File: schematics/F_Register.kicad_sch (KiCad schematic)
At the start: 5 parts, among them U1 74LS377

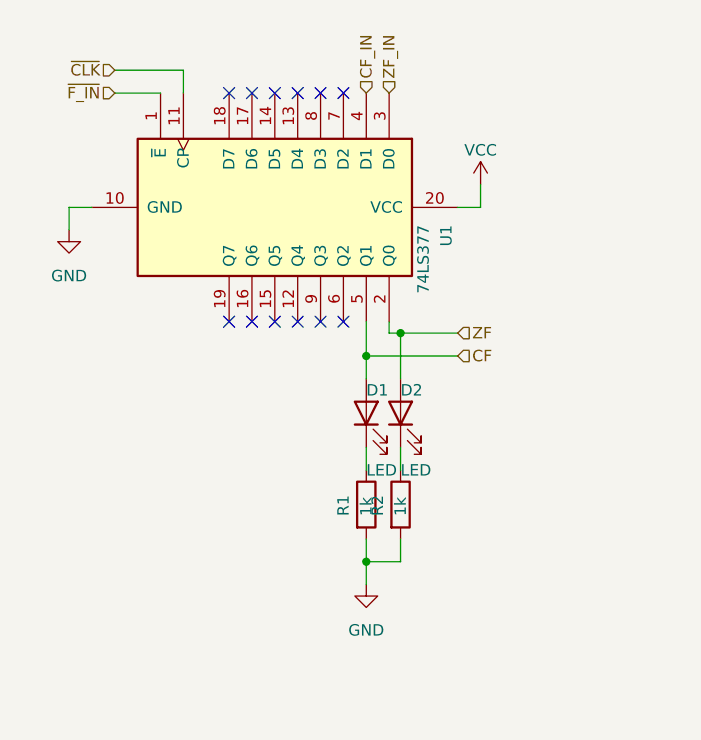
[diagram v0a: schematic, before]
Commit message: E
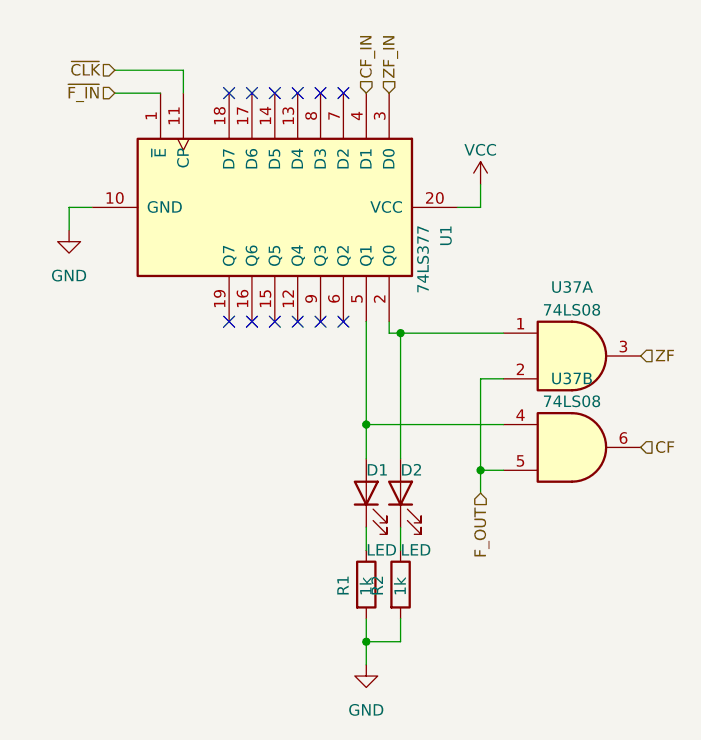
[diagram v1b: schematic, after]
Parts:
- added U37: 74LS08, symbol 74xx:74LS08
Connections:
- net CF: now also U37.6; no longer D1.2 (A), U1.5 (Q1)
- net ZF: now also U37.3; no longer D2.2 (A), U1.2 (Q0)
- new net: D1.2 (A), U1.5 (Q1), U37.4
- new net: D2.2 (A), U1.2 (Q0), U37.1
- new net F_OUT: U37.2, U37.5
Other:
- moved on the sheet: D1, D2, R1, R2
